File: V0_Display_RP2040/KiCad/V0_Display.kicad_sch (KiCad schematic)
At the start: 39 parts, among them J1 GPIO, J2 I2C Header, J2 USB4105-GF-A, J3 SWD, J7 USB_Header, J8 Neopixel, SW6 Kill_SW, SW7 Rotary_Enc, U1 AP2127K-3.3, U2 W25Q16JVUXIQ, U3 74LVC1G17, U4 RP2040, Y1 12MHz

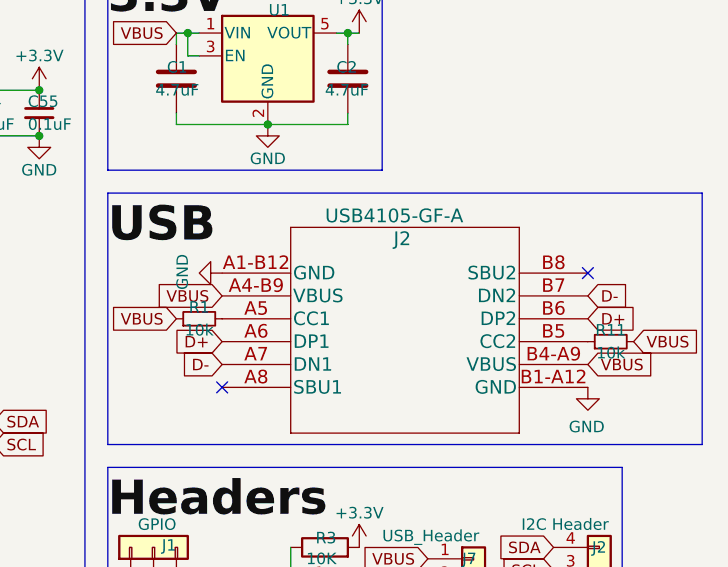
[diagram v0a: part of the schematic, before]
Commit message: Fix Footprints
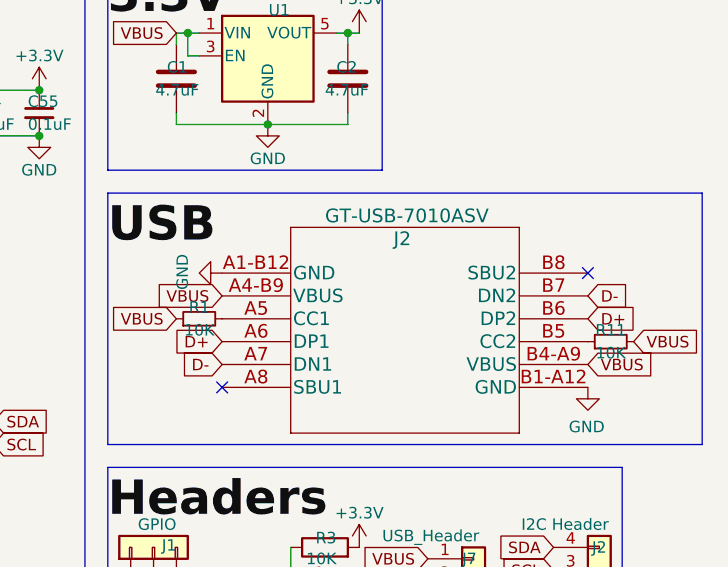
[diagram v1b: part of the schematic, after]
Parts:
- J2: value USB4105-GF-A -> GT-USB-7010ASV; footprint footprints:USB4105-GF-A -> Connector_USB:USB_C_Receptacle_G-Switch_GT-USB-7010ASV
- R1, R11: value 10k -> 10K
- U3: footprint V0-Display:SOT-753 -> Package_TO_SOT_SMD:SOT-23-5
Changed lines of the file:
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@@
       (effects (font (size 1.27 1.27)))
     )
-    (property "Footprint" "V0-Display:SOT-753" (at 111.76 189.23 0)
+    (property "Footprint" "Package_TO_SOT_SMD:SOT-23-5" (at 111.76 189.23 0)
       (effects (font (size 1.27 1.27)) hide)
     )
@@
       (effects (font (size 1.524 1.524)) (justify left))
     )
-    (property "Value" "USB4105-GF-A" (at 118.11 91.44 0)
+    (property "Value" "GT-USB-7010ASV" (at 118.11 91.44 0)
       (effects (font (size 1.524 1.524)) (justify left))
     )
-    (property "Footprint" "footprints:USB4105-GF-A" (at 127 91.694 0)
+    (property "Footprint" "Connector_USB:USB_C_Receptacle_G-Switch_GT-USB-7010ASV" (at 127 91.694 0)
       (effects (font (size 1.524 1.524)) hide)
     )
@@
       (effects (font (size 1.27 1.27)))
     )
-    (property "Value" "10k" (at 149.86 106.68 90)
+    (property "Value" "10K" (at 149.86 106.68 90)
       (effects (font (size 1.27 1.27)))
     )
@@
       (effects (font (size 1.27 1.27)))
     )
-    (property "Value" "10k" (at 104.14 104.14 90)
-      (effects (font (size 1.27 1.27)))
-    )
+    (property "Value" "10K" (at 104.14 104.14 90)
+      (effects (font (size 1.27 1.27)))
+    )
